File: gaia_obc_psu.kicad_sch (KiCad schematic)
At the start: 20 parts, among them J3 Conn_01x02_Pin, Q1 FS8205A, U2 LGS4056H, U3 DW01A, U5 AP2112K-3.3, U8 INA219AxDCN

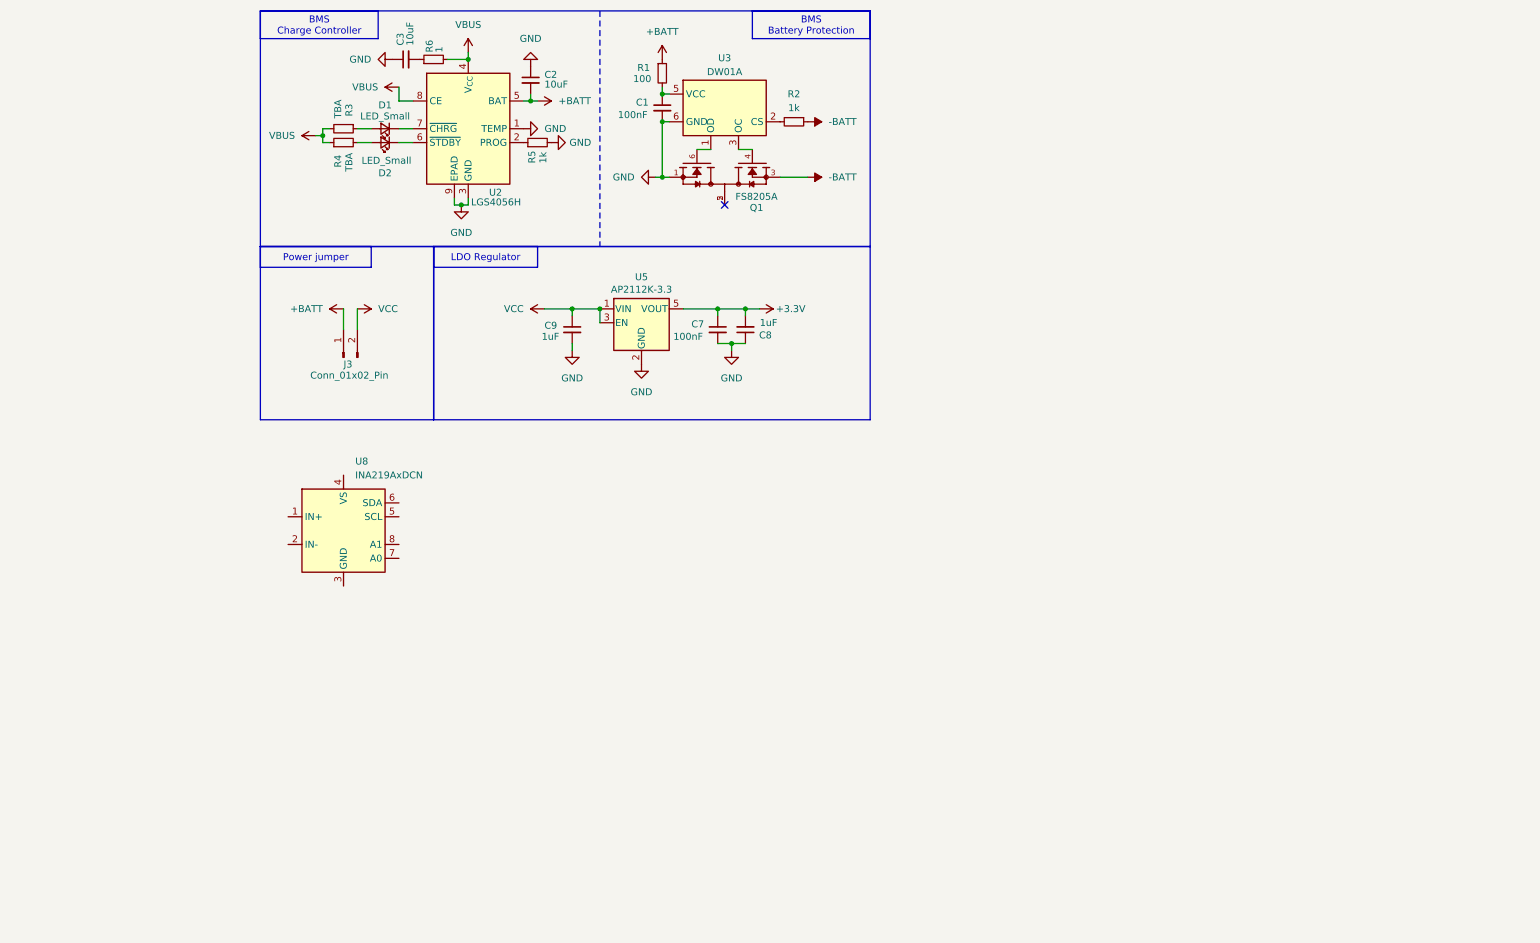
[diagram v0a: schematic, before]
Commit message: preparing ina3221
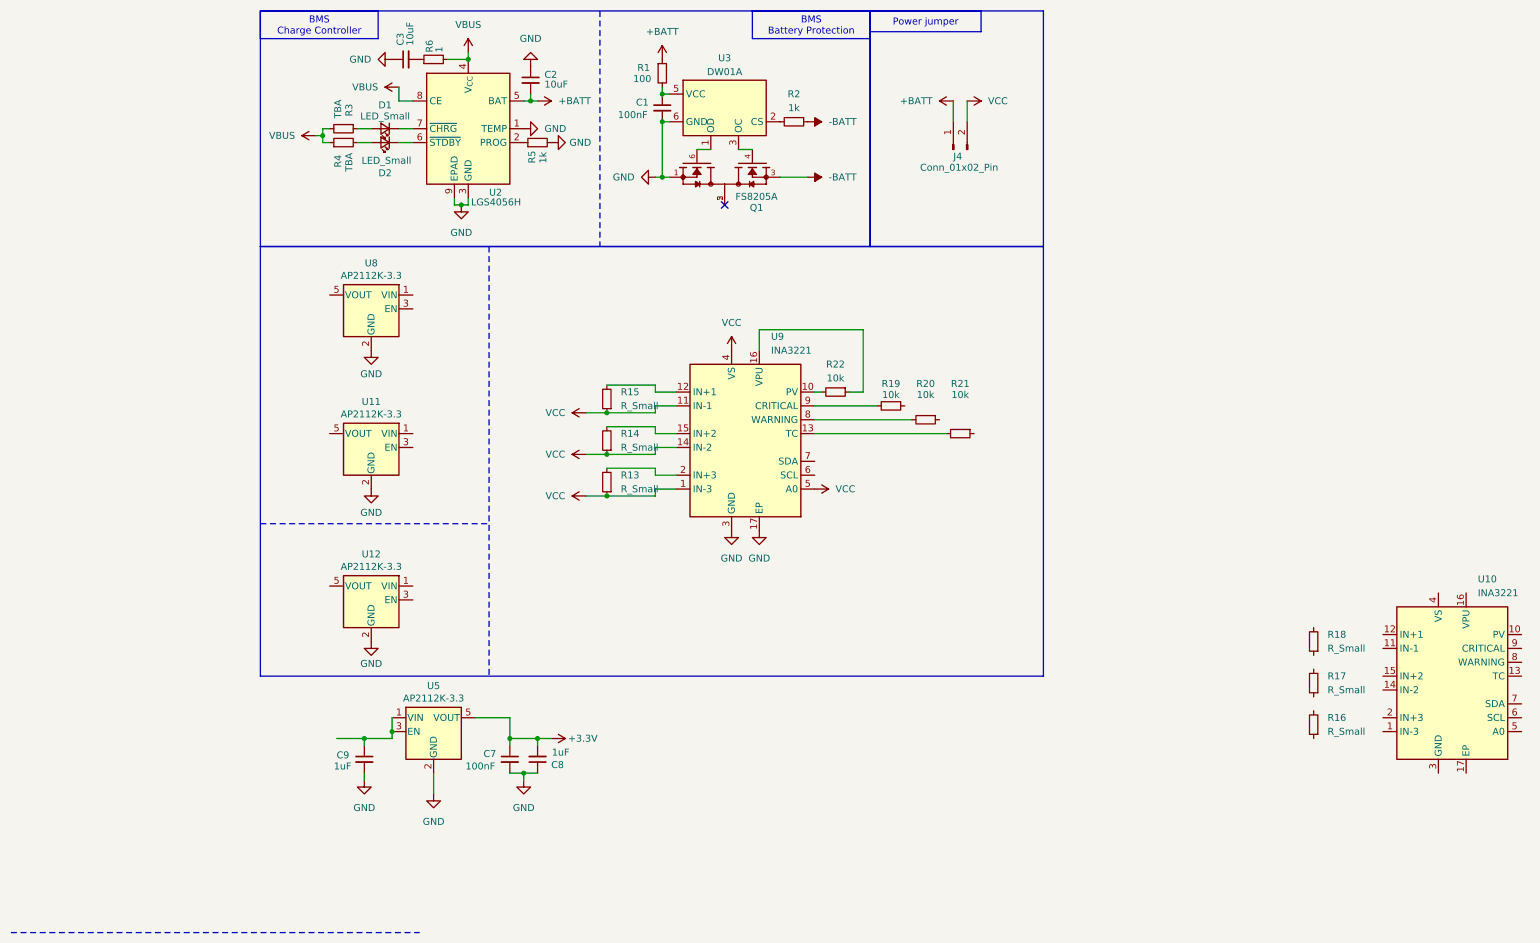
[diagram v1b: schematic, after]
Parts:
- removed J3: Conn_01x02_Pin, Connector_Molex:Molex_MicroClasp_55935-0230_1x02_P2.00mm_Horizontal, symbol Connector:Conn_01x02_Pin
- removed U8: INA219AxDCN, Package_TO_SOT_SMD:SOT-23-8, symbol Sensor_Energy:INA219AxDCN
- added J4: Conn_01x02_Pin, Connector_Molex:Molex_MicroClasp_55935-0230_1x02_P2.00mm_Horizontal, symbol Connector:Conn_01x02_Pin
- added R13, R14, R15, R16, R17, R18: R_Small, symbol Device:R_Small
- added R19, R20, R21, R22: 10k, symbol Device:R_Small
- added U10, U9: INA3221, Package_DFN_QFN:Texas_RGV0016A_VQFN-16-1EP_4x4mm_P0.65mm_EP2.1x2.1mm, symbol Power_Management:INA3221
- added U11, U12, U8: AP2112K-3.3, Package_TO_SOT_SMD:SOT-23-5, symbol Regulator_Linear:AP2112K-3.3
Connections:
- net +BATT: now also J4.1 (Pin_1)
- net GND: now also U11.2 (GND), U12.2 (GND), U8.2 (GND), U9.17 (EP), U9.3 (GND)
- net VCC: now also J4.2 (Pin_2), R13.1, R14.1, R15.1, U9.1 (IN-3), U9.11 (IN-1), U9.14 (IN-2), U9.4 (VS), U9.5 (A0); no longer C9.1, U5.1 (VIN), U5.3 (EN)
- new net: R19.2, U9.9 (CRITICAL)
- new net: R22.2, U9.10 (PV)
- new net: R15.2, U9.12 (IN+1)
- new net: R21.2, U9.13 (TC)
- new net: R14.2, U9.15 (IN+2)
- new net: R22.1, U9.16 (VPU)
- new net: R13.2, U9.2 (IN+3)
- new net: R20.2, U9.8 (WARNING)
- new net: C9.1, U5.1 (VIN), U5.3 (EN)
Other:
- moved on the sheet: C7, C8, C9, U5
